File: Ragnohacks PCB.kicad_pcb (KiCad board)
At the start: 2 copper layers, 85.6 x 54 mm, 35 parts, among them J1 Conn_01x02, J2 Conn_01x18, J3 Conn_01x18, J4 USB_A, SW1 SW_Push, U1 RP2040, U2 W25Q128JVS, U3 LD1117S33TR_SOT223, U4 USBLC6-2P6, Y1 12MHz

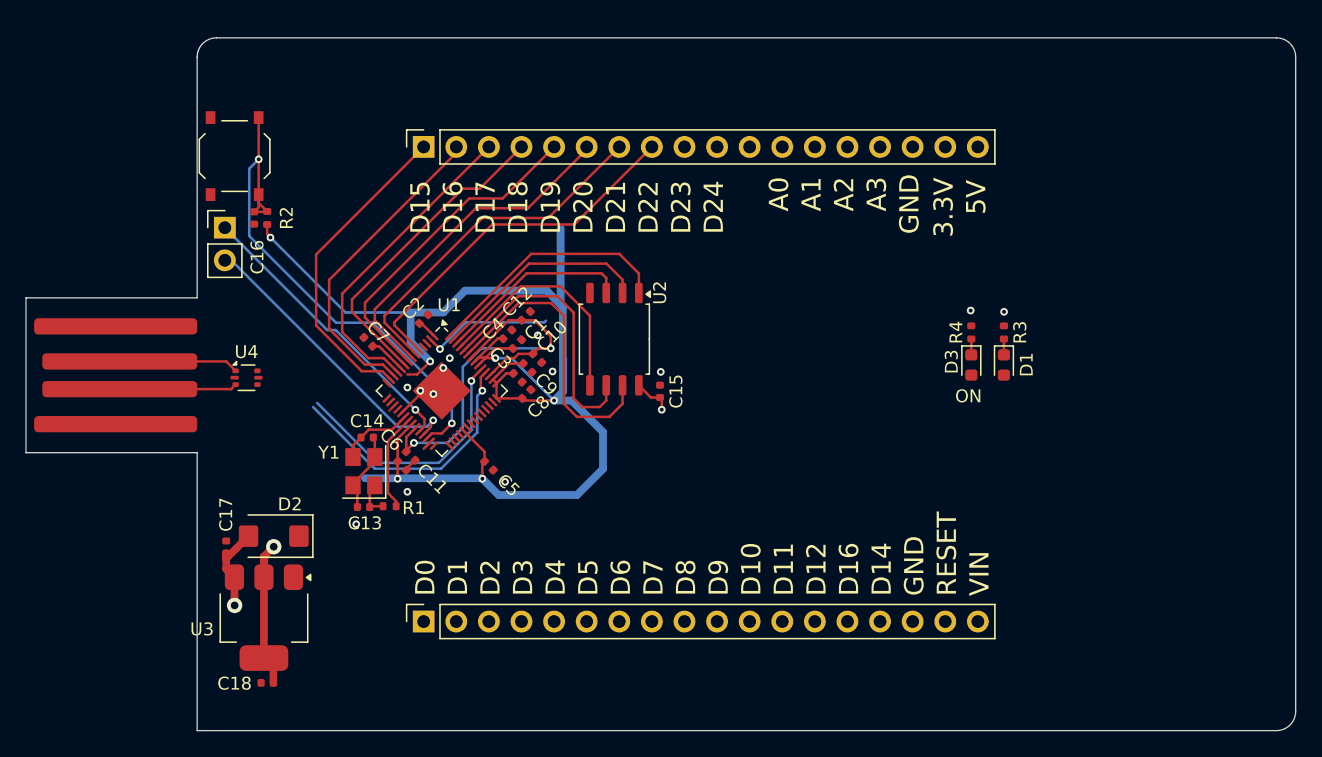
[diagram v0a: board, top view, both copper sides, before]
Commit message: Rev 2 of the Ragnohacks PCB
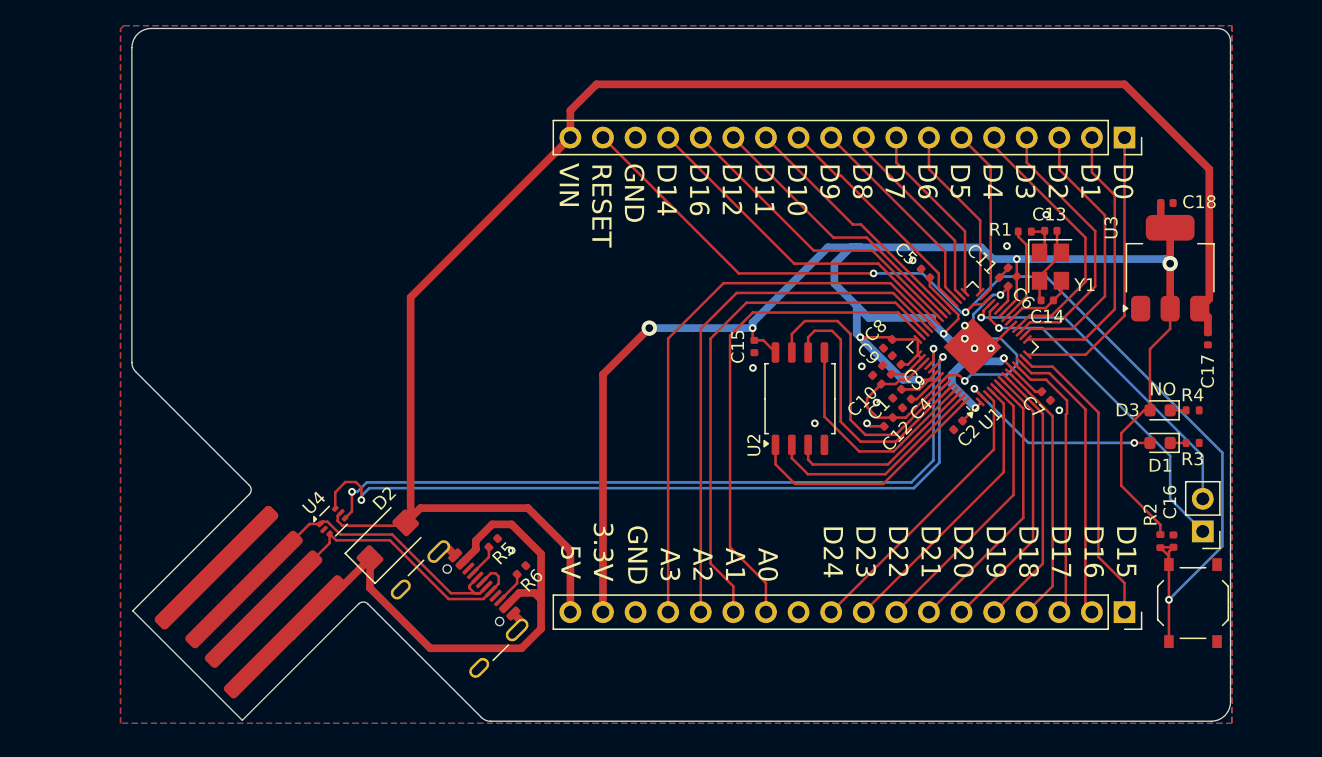
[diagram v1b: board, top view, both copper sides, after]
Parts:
- added J5: USB_C_Receptacle_USB2.0_16P, Connector_USB:USB_C_Receptacle_GCT_USB4105-xx-A_16P_TopMnt_Horizontal, F.Cu at (123.2, 122.7)
- added R5: 5k1, Capacitor_SMD:C_0402_1005Metric, F.Cu at (126.6, 116.8)
- added R6: 5k1, Capacitor_SMD:C_0402_1005Metric, F.Cu at (128.8, 118.9)
- J4: footprint Connector_USB:USB_A_Onboard -> Connector_USB:USB_A_Edge
- moved SW1 82.4 mm to (181.1, 121.4), turned to -90 degrees
- moved J1 79.8 mm to (181.9, 115.9), turned to 180 degrees
- moved C18 79.5 mm to (179.1, 90.3), turned to 0 degrees
- moved C17 78.2 mm to (182.3, 100.8), turned to -90 degrees
- moved C16 75.9 mm to (179.6, 116.6), turned to -90 degrees
- moved U3 75.7 mm to (179.3, 95.4), turned to 90 degrees
- moved R2 74.0 mm to (178.6, 116.6), turned to 90 degrees
- moved J2 66.4 mm to (175.8, 85.2), turned to -90 degrees
- moved J3 65.5 mm to (175.8, 122.2), turned to -90 degrees
- moved C13 57.7 mm to (170.0, 92.4), turned to 180 degrees
- moved Y1 55.8 mm to (170.0, 95.2), turned to -90 degrees
- moved C14 54.1 mm to (169.7, 97.9), turned to 0 degrees
- moved R1 53.9 mm to (168.0, 92.5), turned to 180 degrees
- moved C7 53.0 mm to (169.7, 105.3), turned to -45 degrees
- moved C6 49.9 mm to (167.0, 95.7), turned to 135 degrees
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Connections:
- net Net-(J4-D+) renamed DN
- net Net-(J4-D-) renamed DP
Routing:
- net +5V: track 7.20 -> 129.9 mm, vias 1 -> 0
- net Net-(D2-A): track 0.00 -> 45.2 mm
- net A3: track 0.00 -> 45.0 mm
- net RESET: track 41.6 -> 86.1 mm, vias 2 -> 3
- net A2: track 0.00 -> 42.1 mm
- net A1: track 0.00 -> 40.9 mm
- net USB_DP: track 20.1 -> 60.9 mm, vias 1 -> 2
- net A0: track 0.00 -> 39.1 mm
- net USB_DN: track 21.0 -> 58.8 mm, vias 1 -> 2
- net +3V3: track 132.3 -> 169.1 mm, vias 8 -> 9
- net D14: track 0.00 -> 26.8 mm
- net D13: track 0.00 -> 24.4 mm
- net D0: track 0.00 -> 22.7 mm
- net D24: track 0.00 -> 22.4 mm
- net D23: track 0.00 -> 22.2 mm
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- added copper zone on B.Cu, net GND
- added copper zone on F.Cu, net GND
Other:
- outline, holes or cut-outs redrawn
